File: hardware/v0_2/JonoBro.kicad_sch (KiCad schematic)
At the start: 65 parts, among them J1 Conn_01x02_Pin, J2 Conn_01x02_Pin, J3 Conn_01x02_Pin, J3 USB_C_Receptacle_USB2.0, J4 Conn_01x02_Pin, Q1 CSD19537Q3, Q10 CSD19537Q3, Q2 MMBT3904, Q3 CSD19537Q3, Q4 MMBT3904, Q5 CSD19537Q3, Q6 CSD19537Q3, Q7 MMBT3904, Q8 CSD19537Q3, Q9 CSD19537Q3, SW1 SW_Push, SW2 SW_Push, U2 ESP32-C3-MINI-1, U3 AOZ1280CI

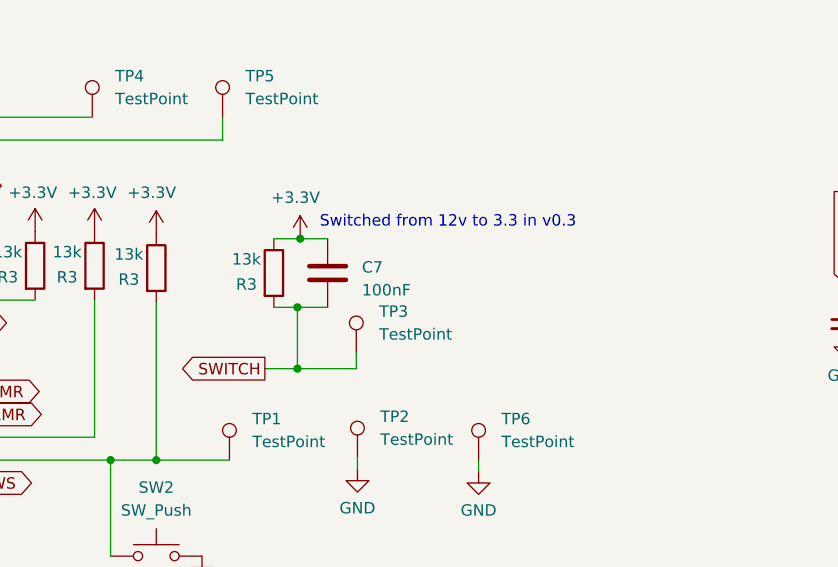
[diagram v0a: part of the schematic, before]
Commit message: board updates
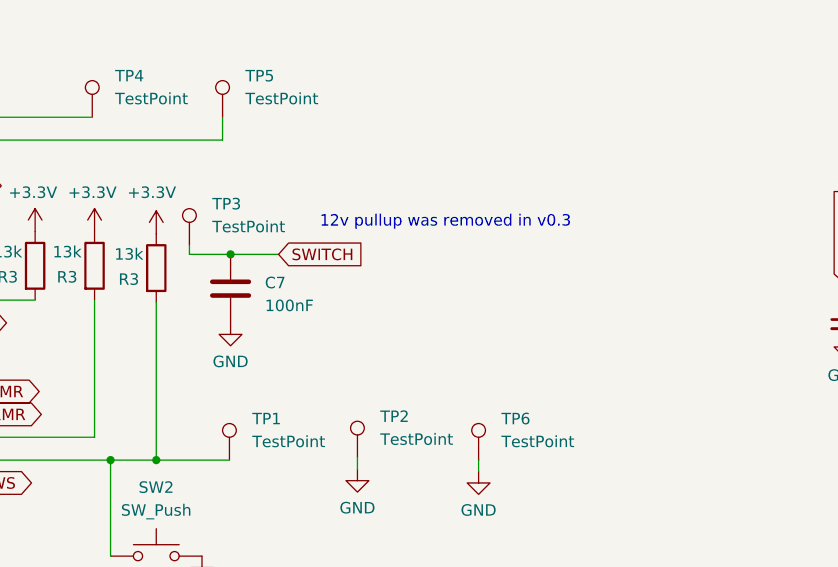
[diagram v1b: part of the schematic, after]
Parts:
- removed R3: 13k, Resistor_SMD:R_0603_1608Metric, symbol Device:R
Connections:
- net +3.3V: no longer C7.1
- net GND: now also C7.2
- net SWITCH: now also C7.1; no longer C7.2
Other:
- note added: "12v pullup was removed in v0.3"
- note removed: "Switched from 12v to 3.3 in v0.3"
- moved on the sheet: C7, TP3
